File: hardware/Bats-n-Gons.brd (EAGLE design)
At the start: 85.7 x 65.1 mm, 49 parts, among them SW1 SMD_SWITCH, U1 SAMD51PXXA, U2 IS31AP4991, X4 32.768

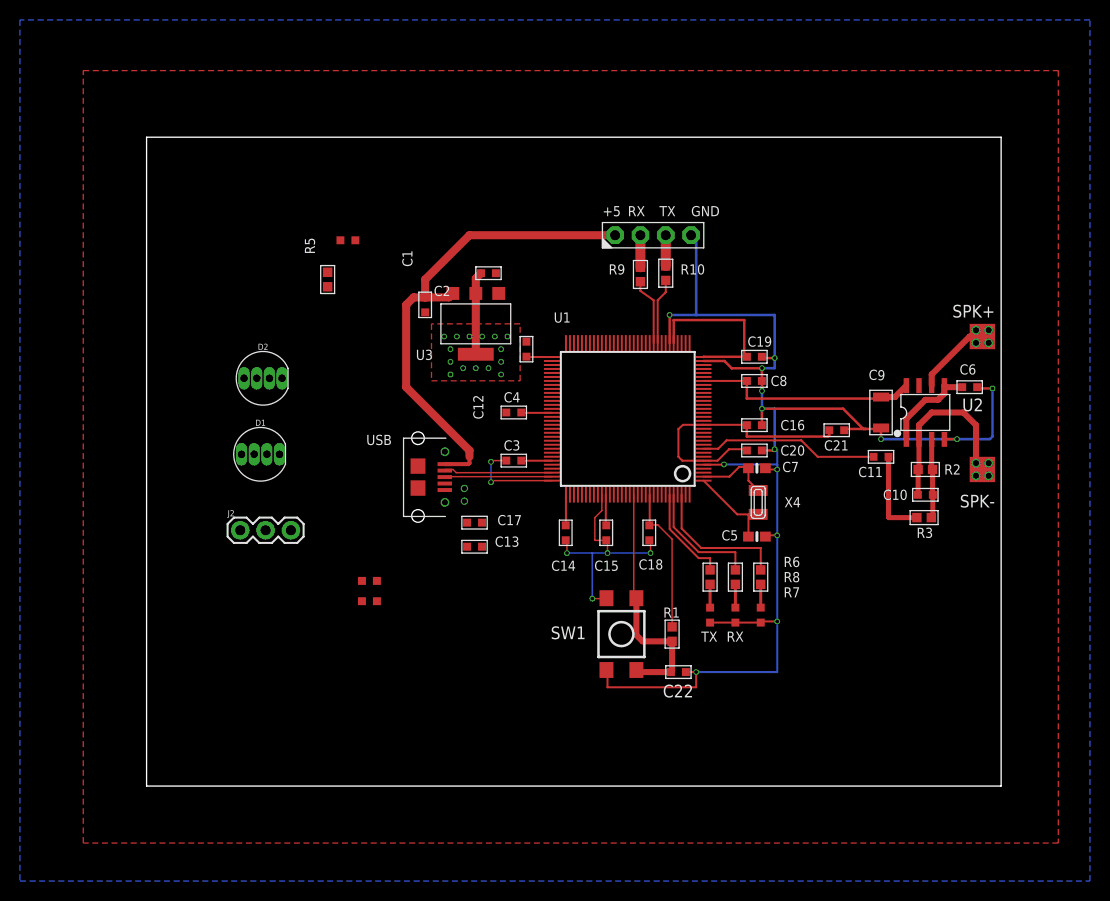
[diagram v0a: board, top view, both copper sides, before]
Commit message: maybe good enough for 0.0
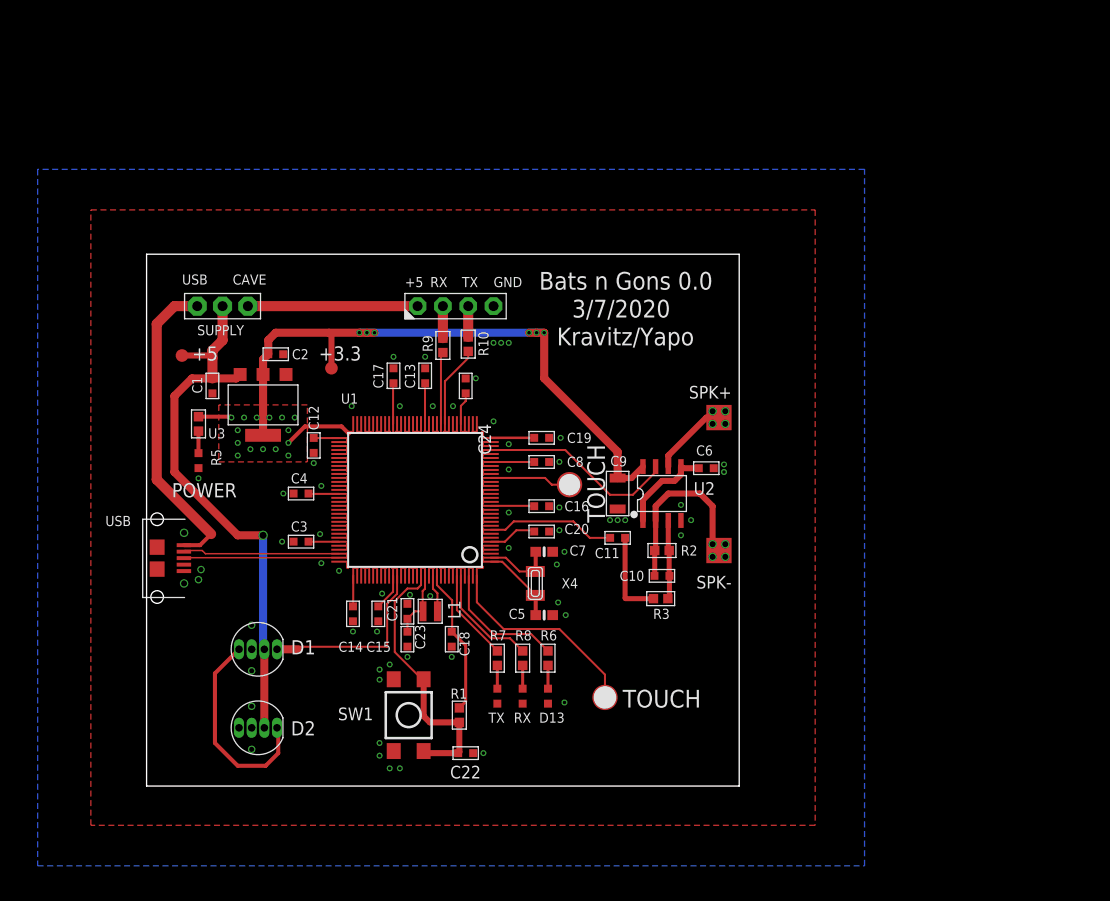
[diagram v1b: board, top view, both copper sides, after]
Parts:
- removed D13_LED1, PWR_LED1: (no value), bats-n-gons:LED_0603
- removed J2: (no value), SparkFun-Connectors:1X03
- added C23: 0.1u, bats-n-gons:C0603
- added C24: (no value), bats-n-gons:C0603
- added L1: 10u, bats-n-gons:L24X24
- added PAD_TOUCH, PAD_TOUCH1: PAD, bats-n-gons:PAD-ROUND-100MIL-MASK
- added U$1: HEADER_3PIN, bats-n-gons:HEADER_3PIN
- added U$33, U$34: PADROUND-50MIL, bats-n-gons:PAD-ROUND-50MIL
- C21: value (none) -> 10u
- D1, D2: value DIFFUSE -> (none); device SparkFun-LED:LED-RGB-THRU -> bats-n-gons:LED-RGB-THRU
- moved C21 46.7 mm to (26.2, 17.5), turned to 270 degrees
- moved D2 35.1 mm to (11.2, 5.84)
- moved C10 27.6 mm to (51.7, 21.1)
- moved R2 27.6 mm to (51.7, 23.6)
- moved U2 27.6 mm to (51.7, 29.3)
- moved C11 27.6 mm to (47.2, 24.9)
- moved C6 27.6 mm to (56.1, 31.9)
- moved C9 27.6 mm to (47.2, 29.3)
- moved R3 27.6 mm to (51.6, 18.8)
- moved SPK+ 27.6 mm to (57.4, 37.0)
- moved SPK- 27.6 mm to (57.4, 23.6)
- moved USB 27.4 mm to (0.00, 27.9)
- moved PWR_LED 26.7 mm to (5.21, 32.6), turned to 270 degrees
- moved C15 24.3 mm to (23.2, 17.3)
- moved X4 23.8 mm to (39.0, 20.3)
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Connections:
- net N$6 renamed !RESET!
- new net N$15: U$1.3, USB.VBUS
- new net N$16: J1.1, U$1.1
- new net N$17: D1.4, D2.1
- new net N$18: C21.P$2, C23.P$2, L1.1, U1.115
- new net N$19: L1.2, U1.117
- net +3.3V: now also C24.P$2, U$33.P$1; no longer C21.P$2
- net +5V: now also D1.2, D2.2, U$1.2, U$34.P$1; no longer J1.1, J2.3, USB.VBUS
- net A1: now also PAD_TOUCH1.P$1
- net A2: now also PAD_TOUCH.P$1
- net D2: no longer U2.7
- net D46: now also U2.7
- net GND: now also C23.P$1, C24.P$1, D1.3, D2.3
- net NEOPIX: now also D1.1
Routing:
- net GND: track 178.8 -> 1.43 mm, vias 22 -> 61
- net N$15: track 0.00 -> 31.3 mm
- net +3.3V: track 105.8 -> 135.5 mm, vias 15 -> 21
- net N$17: track 0.00 -> 20.8 mm
- net A2: track 0.00 -> 20.8 mm
- net D46: track 0.00 -> 19.9 mm
- net NEOPIX: track 0.00 -> 18.7 mm
- net N$16: track 0.00 -> 17.0 mm
- net A1: track 0.00 -> 8.17 mm
- net +5V: track 48.9 -> 56.8 mm, vias 0 -> 1
- net N$18: track 0.00 -> 6.86 mm
- net A0: track 18.1 -> 13.0 mm
- net D+: track 10.8 -> 15.6 mm
- net D-: track 10.9 -> 15.8 mm
- net N$19: track 0.00 -> 3.76 mm
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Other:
- board size 85.7 x 65.1 mm -> 59.4 x 53.3 mm
- board text added: "+3.3"
- board text added: "3/7/2020"
- board text added: "Bats n Gons 0.0"
- board text added: "CAVE"
- board text added: "D1"
- board text added: "D13"
- board text added: "D2"
- board text added: "Kravitz/Yapo"
- board text added: "POWER"
- board text added: "SUPPLY"
- board text added: "TOUCH"
- board text added: "USB"
